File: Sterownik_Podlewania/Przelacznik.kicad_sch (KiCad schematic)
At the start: 3 parts, among them SW2 SW_Nidec_CAS-120A1

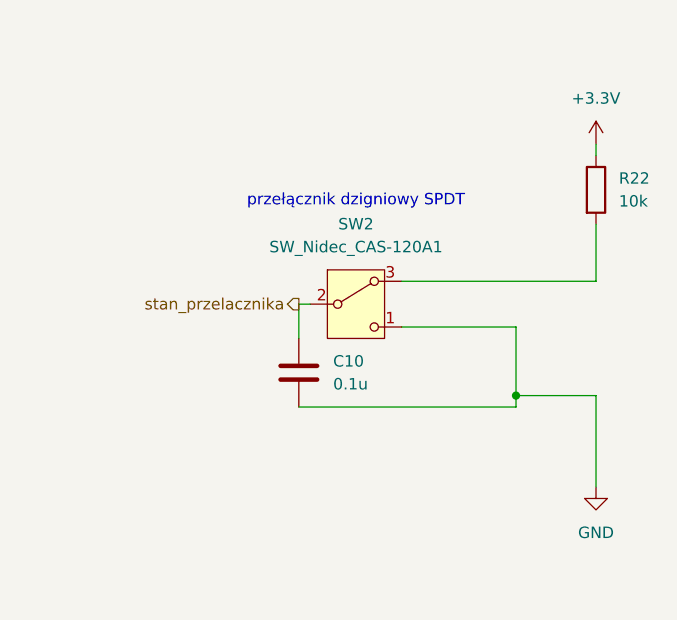
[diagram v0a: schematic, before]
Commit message: Poprawki estetyczne schematu
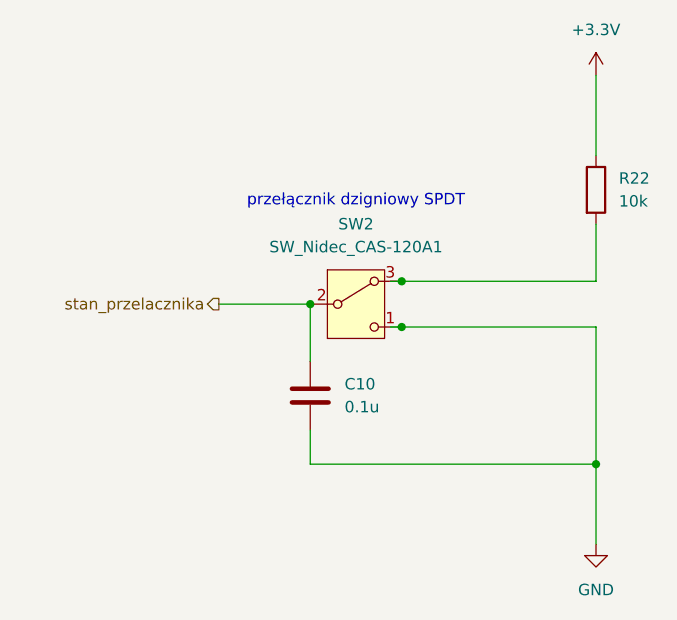
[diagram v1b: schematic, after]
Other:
- moved on the sheet: C10
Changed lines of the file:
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@@
 	)
 	(junction
-		(at 156.21 109.22)
+		(at 143.51 96.52)
 		(diameter 0)
 		(color 0 0 0 0)
 	)
-	(wire
-		(pts
-			(xy 165.1 119.38) (xy 165.1 109.22)
-		)
-		(stroke
-			(width 0)
-			(type default)
-		)
-	)
-	(wire
-		(pts
-			(xy 133.35 99.06) (xy 132.08 99.06)
-		)
-		(stroke
-			(width 0)
-			(type default)
-		)
-	)
-	(wire
-		(pts
-			(xy 156.21 101.6) (xy 156.21 109.22)
+	(junction
+		(at 165.1 116.84)
+		(diameter 0)
+		(color 0 0 0 0)
+	)
+	(junction
+		(at 133.35 99.06)
+		(diameter 0)
+		(color 0 0 0 0)
+	)
+	(junction
+		(at 143.51 101.6)
+		(diameter 0)
+		(color 0 0 0 0)
+	)
+	(wire
+		(pts
+			(xy 133.35 99.06) (xy 123.19 99.06)
 		)
 		(stroke
@@
 	(wire
 		(pts
-			(xy 156.21 109.22) (xy 165.1 109.22)
+			(xy 143.51 101.6) (xy 165.1 101.6)
+		)
+		(stroke
+			(width 0)
+			(type default)
+		)
+	)
+	(wire
+		(pts
+			(xy 142.24 101.6) (xy 143.51 101.6)
+		)
+		(stroke
+			(width 0)
+			(type default)
+		)
+	)
+	(wire
+		(pts
+			(xy 133.35 113.03) (xy 133.35 116.84)
 		)
 		(stroke
@@
 	(wire
 		(pts
-			(xy 132.08 110.49) (xy 156.21 110.49)
-		)
-		(stroke
-			(width 0)
-			(type default)
-		)
-	)
-	(wire
-		(pts
-			(xy 143.51 101.6) (xy 156.21 101.6)
-		)
-		(stroke
-			(width 0)
-			(type default)
-		)
-	)
-	(wire
-		(pts
-			(xy 132.08 99.06) (xy 132.08 102.87)
-		)
-		(stroke
-			(width 0)
-			(type default)
-		)
-	)
-	(wire
-		(pts
-			(xy 165.1 81.28) (xy 165.1 82.55)
-		)
-		(stroke
-			(width 0)
-			(type default)
-		)
-	)
-	(wire
-		(pts
-			(xy 156.21 110.49) (xy 156.21 109.22)
+			(xy 142.24 96.52) (xy 143.51 96.52)
+		)
+		(stroke
+			(width 0)
+			(type default)
+		)
+	)
+	(wire
+		(pts
+			(xy 165.1 101.6) (xy 165.1 116.84)
+		)
+		(stroke
+			(width 0)
+			(type default)
+		)
+	)
+	(wire
+		(pts
+			(xy 133.35 99.06) (xy 133.35 105.41)
+		)
+		(stroke
+			(width 0)
+			(type default)
+		)
+	)
+	(wire
+		(pts
+			(xy 133.35 116.84) (xy 165.1 116.84)
+		)
+		(stroke
+			(width 0)
+			(type default)
+		)
+	)
+	(wire
+		(pts
+			(xy 165.1 73.66) (xy 165.1 82.55)
+		)
+		(stroke
+			(width 0)
+			(type default)
+		)
+	)
+	(wire
+		(pts
+			(xy 165.1 116.84) (xy 165.1 125.73)
 		)
 		(stroke
@@
 	(hierarchical_label "stan_przelacznika"
 		(shape output)
-		(at 132.08 99.06 180)
+		(at 123.19 99.06 180)
 		(effects
 			(font
@@
 			)
 			(justify right)
-		)
-	)
-	(rule_area
-		(polyline
-			(pts
-				(xy 179.705 72.7074) (xy 179.07 126.365) (xy 111.76 125.73) (xy 111.76 72.39)
-			)
-			(stroke
-				(width 0)
-				(type dash)
-			)
-			(fill
-				(type none)
-			)
 		)
 	)
@@
 					(unit 1)
 				)
+				(path "/a66bdf1f-0e2a-4cc5-beb1-605f2a3b9885/9a88e80e-3101-4c9e-b6e9-f6fd66520dd2/adff730d-5353-4d94-b665-43238fb73228"
+					(reference "R14")
+					(unit 1)
+				)
 				(path "/a66bdf1f-0e2a-4cc5-beb1-605f2a3b9885/aaafd38c-ffc0-4fc7-936b-5b26ec62426f/568b4e0a-513a-44c1-8d45-ad0443c3ee4b"
 					(reference "R24")
@@
 	(symbol
 		(lib_id "power:GND")
-		(at 165.1 119.38 0)
+		(at 165.1 125.73 0)
 		(unit 1)
 		(exclude_from_sim no)
@@
 		(fields_autoplaced yes)
 		(property "Reference" "#PWR063"
+			(at 165.1 132.08 0)
+			(effects
+				(font
+					(size 1.27 1.27)
+				)
+				(hide yes)
+			)
+		)
+		(property "Value" "GND"
+			(at 165.1 130.81 0)
+			(effects
+				(font
+					(size 1.27 1.27)
+				)
+			)
+		)
+		(property "Footprint" ""
 			(at 165.1 125.73 0)
 			(effects
@@
 			)
 		)
-		(property "Value" "GND"
-			(at 165.1 124.46 0)
-			(effects
-				(font
-					(size 1.27 1.27)
-				)
-			)
-		)
-		(property "Footprint" ""
-			(at 165.1 119.38 0)
-			(effects
-				(font
-					(size 1.27 1.27)
-				)
-				(hide yes)
-			)
-		)
 		(property "Datasheet" ""
-			(at 165.1 119.38 0)
+			(at 165.1 125.73 0)
 			(effects
 				(font
@@
 		)
 		(property "Description" "Power symbol creates a global label with name \"GND\" , ground"
-			(at 165.1 119.38 0)
+			(at 165.1 125.73 0)
 			(effects
 				(font
@@
 					(unit 1)
 				)
+				(path "/a66bdf1f-0e2a-4cc5-beb1-605f2a3b9885/9a88e80e-3101-4c9e-b6e9-f6fd66520dd2/adff730d-5353-4d94-b665-43238fb73228"
+					(reference "#PWR044")
+					(unit 1)
+				)
 				(path "/a66bdf1f-0e2a-4cc5-beb1-605f2a3b9885/aaafd38c-ffc0-4fc7-936b-5b26ec62426f/568b4e0a-513a-44c1-8d45-ad0443c3ee4b"
 					(reference "#PWR067")
@@
 	(symbol
 		(lib_id "Device:C")
-		(at 132.08 106.68 0)
+		(at 133.35 109.22 0)
 		(unit 1)
 		(exclude_from_sim no)
@@
 		(fields_autoplaced yes)
 		(property "Reference" "C10"
-			(at 135.89 105.4099 0)
+			(at 137.16 107.9499 0)
 			(effects
 				(font
@@
 		)
 		(property "Value" "0.1u"
-			(at 135.89 107.9499 0)
+			(at 137.16 110.4899 0)
 			(effects
 				(font
@@
 		)
 		(property "Footprint" "Capacitor_SMD:C_1206_3216Metric"
-			(at 133.0452 110.49 0)
+			(at 134.3152 113.03 0)
 			(effects
 				(font
@@
 		)
 		(property "Datasheet" "~"
-			(at 132.08 106.68 0)
+			(at 133.35 109.22 0)
 			(effects
 				(font
@@
 		)
 		(property "Description" "Unpolarized capacitor"
-			(at 132.08 106.68 0)
+			(at 133.35 109.22 0)
 			(effects
 				(font
@@
 					(unit 1)
 				)
+				(path "/a66bdf1f-0e2a-4cc5-beb1-605f2a3b9885/9a88e80e-3101-4c9e-b6e9-f6fd66520dd2/adff730d-5353-4d94-b665-43238fb73228"
+					(reference "C1")
+					(unit 1)
+				)
 				(path "/a66bdf1f-0e2a-4cc5-beb1-605f2a3b9885/aaafd38c-ffc0-4fc7-936b-5b26ec62426f/568b4e0a-513a-44c1-8d45-ad0443c3ee4b"
 					(reference "C12")
@@
 	(symbol
 		(lib_id "power:+5V")
-		(at 165.1 81.28 0)
+		(at 165.1 73.66 0)
 		(unit 1)
 		(exclude_from_sim no)
@@
 		(fields_autoplaced yes)
 		(property "Reference" "#PWR062"
-			(at 165.1 85.09 0)
+			(at 165.1 77.47 0)
 			(effects
 				(font
@@
 		)
 		(property "Value" "+3.3V"
-			(at 165.1 76.2 0)
+			(at 165.1 68.58 0)
 			(effects
 				(font
@@
 		)
 		(property "Footprint" ""
-			(at 165.1 81.28 0)
+			(at 165.1 73.66 0)
 			(effects
 				(font
@@
 		)
 		(property "Datasheet" ""
-			(at 165.1 81.28 0)
+			(at 165.1 73.66 0)
 			(effects
 				(font
@@
 		)
 		(property "Description" "Power symbol creates a global label with name \"+5V\""
-			(at 165.1 81.28 0)
+			(at 165.1 73.66 0)
 			(effects
 				(font
@@
 				(path "/a66bdf1f-0e2a-4cc5-beb1-605f2a3b9885/995f053e-6bfd-4935-9460-d34c9e8248bd/568b4e0a-513a-44c1-8d45-ad0443c3ee4b"
 					(reference "#PWR070")
+					(unit 1)
+				)
+				(path "/a66bdf1f-0e2a-4cc5-beb1-605f2a3b9885/9a88e80e-3101-4c9e-b6e9-f6fd66520dd2/adff730d-5353-4d94-b665-43238fb73228"
+					(reference "#PWR043")
 					(unit 1)
 				)
@@
 					(unit 1)
 				)
+				(path "/a66bdf1f-0e2a-4cc5-beb1-605f2a3b9885/9a88e80e-3101-4c9e-b6e9-f6fd66520dd2/adff730d-5353-4d94-b665-43238fb73228"
+					(reference "SW9")
+					(unit 1)
+				)
